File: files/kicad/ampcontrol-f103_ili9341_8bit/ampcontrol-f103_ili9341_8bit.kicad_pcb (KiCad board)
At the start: 2 copper layers, 94.4 x 64.8 mm, 61 parts, among them J1 Audio, J10 Buttons, J11 Encoder, J12 TFT, J13 I2C_Audio, J14 I2C_Tuner, J15 I2C_Ext, J2 MUTE_STBY, J3 UART, J4 USB, J5 UART2, J6 UART3, J7 RC, J8 BOOT, J9 5V, SW1 Reset, U1 MCP602, U2 STM32F103CBTx, U3 AMS1117-3.3, Y1 8MHz, Y2 32768

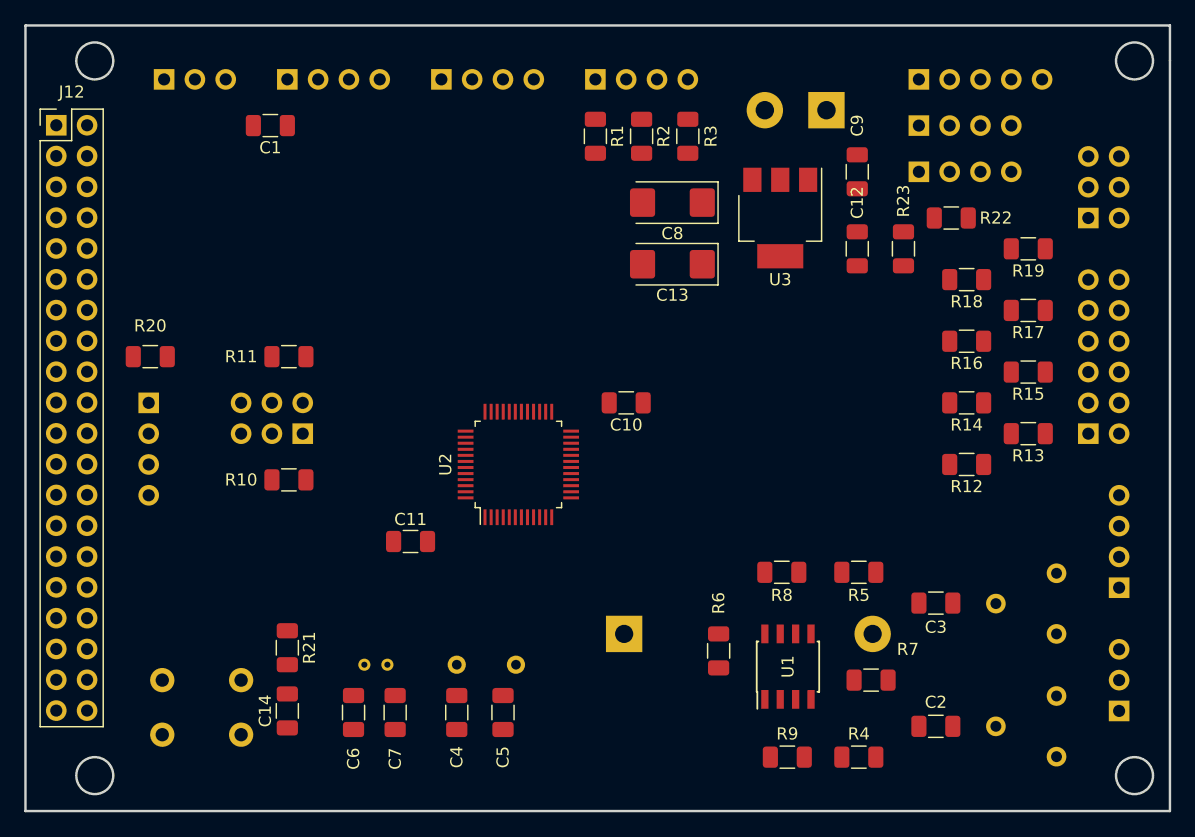
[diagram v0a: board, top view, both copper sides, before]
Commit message: Testing autorouted board
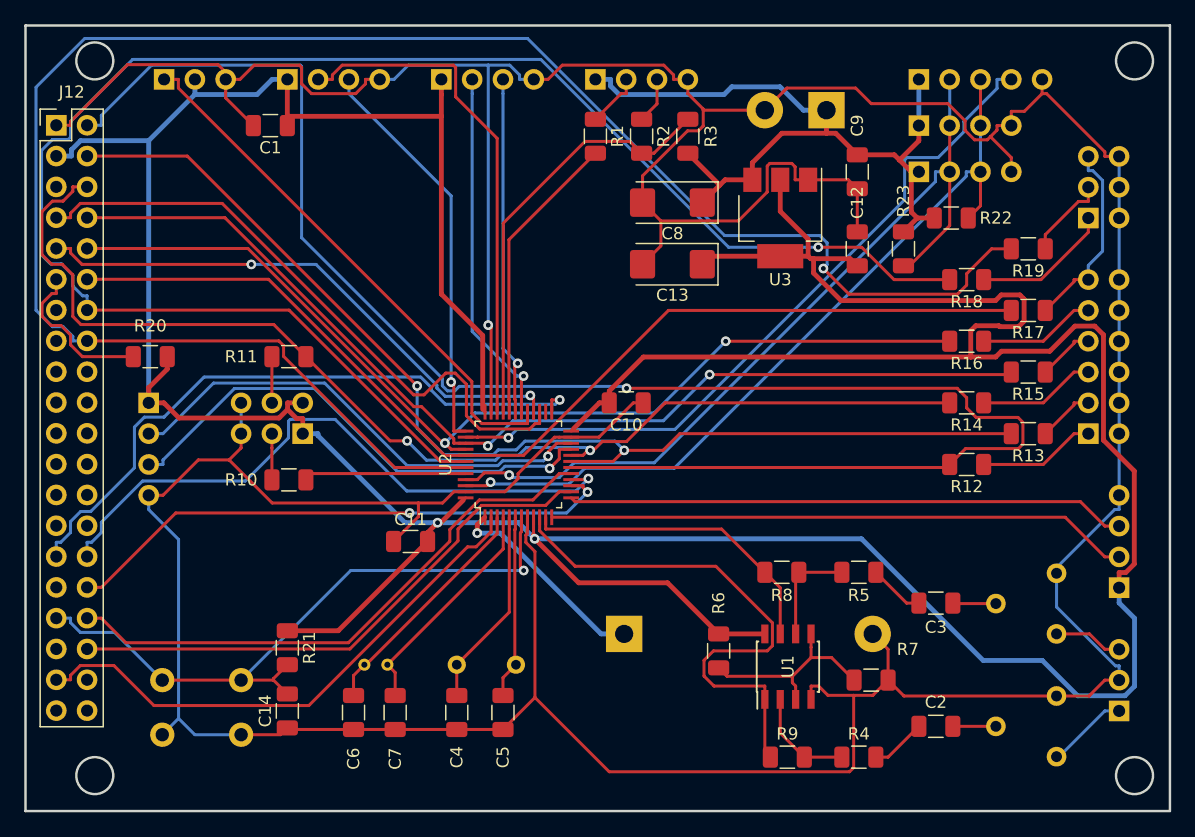
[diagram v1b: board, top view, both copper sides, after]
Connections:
- net Net-(BT1-Pad1) renamed /VBAT
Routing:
- net GNDD: track 0.00 -> 424.8 mm, vias 0 -> 1
- net +3V3: track 0.00 -> 362.2 mm, vias 0 -> 2
- net /DB7: track 0.00 -> 154.5 mm, vias 0 -> 1
- net /DB0: track 0.00 -> 141.2 mm, vias 0 -> 1
- net /DB6: track 0.00 -> 138.1 mm, vias 0 -> 1
- net /DB2: track 0.00 -> 96.1 mm, vias 0 -> 2
- net /DB1: track 0.00 -> 94.5 mm, vias 0 -> 2
- net /DB5: track 0.00 -> 87.2 mm
- net /DB3: track 0.00 -> 86.7 mm, vias 0 -> 2
- net /DB4: track 0.00 -> 83.2 mm, vias 0 -> 2
- net /SCL: track 0.00 -> 68.5 mm, vias 0 -> 1
- net /SDA: track 0.00 -> 65.4 mm, vias 0 -> 1
- net +5V: track 0.00 -> 63.3 mm
- net /HW_RST: track 0.00 -> 60.1 mm, vias 0 -> 1
- net /NRST: track 0.00 -> 55.2 mm, vias 0 -> 1
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- added copper zone on B.Cu, net GNDD
- added copper zone on F.Cu, net GNDD
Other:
- net class Power added: clearance 0.2, trace_width 0.4, via_dia 0.8, via_drill 0.4
